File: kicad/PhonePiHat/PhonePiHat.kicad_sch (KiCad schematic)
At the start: 13 parts, among them J1 Raspberry_Pi_4, J2 Screw_Terminal_01x13, Q1 IRF540N

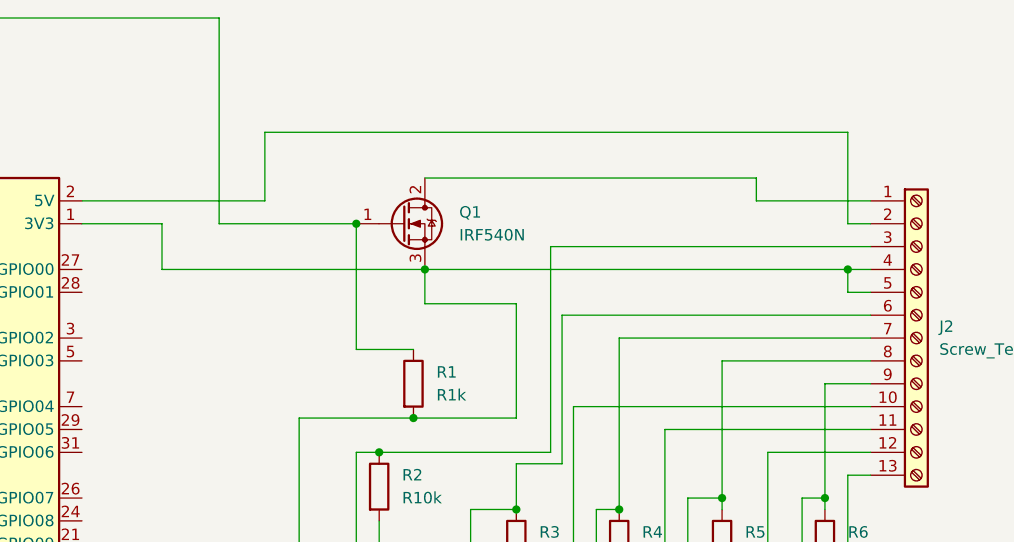
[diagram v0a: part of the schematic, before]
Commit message: v2 board
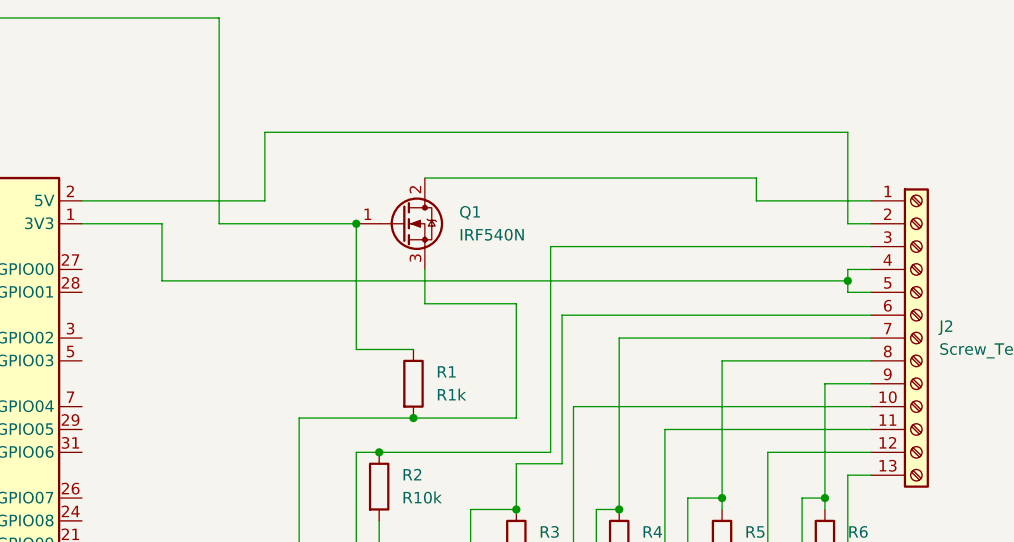
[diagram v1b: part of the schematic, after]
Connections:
- net at J1.14 (GND), J1.20 (GND), J1.25 (GND)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: no longer J1.1 (3V3), J1.17 (3V3), J2.4 (Pin_4), J2.5 (Pin_5)
- new net: J1.1 (3V3), J1.17 (3V3), J2.4 (Pin_4), J2.5 (Pin_5)
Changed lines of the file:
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@@
+	)
+	(junction
+		(at 195.58 49.53)
+		(diameter 0)
+		(color 0 0 0 0)
 	)
 	(junction
@@
 	)
 	(junction
-		(at 195.58 48.26)
-		(diameter 0)
-		(color 0 0 0 0)
-	)
-	(junction
 		(at 193.04 73.66)
 		(diameter 0)
@@
 	)
 	(junction
-		(at 148.59 48.26)
-		(diameter 0)
-		(color 0 0 0 0)
-	)
-	(junction
 		(at 181.61 73.66)
 		(diameter 0)
@@
 	(wire
 		(pts
-			(xy 119.38 48.26) (xy 119.38 43.18)
-		)
-		(stroke
-			(width 0)
-			(type default)
-		)
-	)
-	(wire
-		(pts
 			(xy 195.58 71.12) (xy 195.58 87.63)
 		)
@@
 	(wire
 		(pts
+			(xy 195.58 49.53) (xy 195.58 50.8)
+		)
+		(stroke
+			(width 0)
+			(type default)
+		)
+	)
+	(wire
+		(pts
 			(xy 181.61 82.55) (xy 193.04 82.55)
 		)
@@
 	(wire
 		(pts
-			(xy 195.58 48.26) (xy 148.59 48.26)
-		)
-		(stroke
-			(width 0)
-			(type default)
-		)
-	)
-	(wire
-		(pts
 			(xy 181.61 73.66) (xy 177.8 73.66)
 		)
@@
 	(wire
 		(pts
+			(xy 119.38 43.18) (xy 119.38 49.53)
+		)
+		(stroke
+			(width 0)
+			(type default)
+		)
+	)
+	(wire
+		(pts
 			(xy 143.51 68.58) (xy 162.56 68.58)
 		)
@@
 	(wire
 		(pts
-			(xy 148.59 48.26) (xy 119.38 48.26)
-		)
-		(stroke
-			(width 0)
-			(type default)
-		)
-	)
-	(wire
-		(pts
 			(xy 158.75 52.07) (xy 148.59 52.07)
 		)
@@
 	(wire
 		(pts
-			(xy 195.58 48.26) (xy 195.58 50.8)
+			(xy 195.58 48.26) (xy 195.58 49.53)
 		)
 		(stroke
@@
 		)
 		(stroke
+			(width 0)
+			(type default)
+		)
+	)
+	(wire
+		(pts
+			(xy 119.38 49.53) (xy 195.58 49.53)
+		)
+		(stroke
